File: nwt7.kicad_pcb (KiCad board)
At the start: 2 copper layers, 118.4 x 117.3 mm, 125 parts, among them IC1 PIC16F876A, IC10 AD8307, IC11 MSA0886, IC12 78L10, IC13 AP1117D50, IC15 AP1117D50, IC16 AD8361, IC2 MAX232, IC4 AP1117D50, IC5 AP1117D50, IC6 AD9851, IC7 MSA0886, IC8 7808, IC9 AD8307, Q1 10 MHz, T1 Coupler

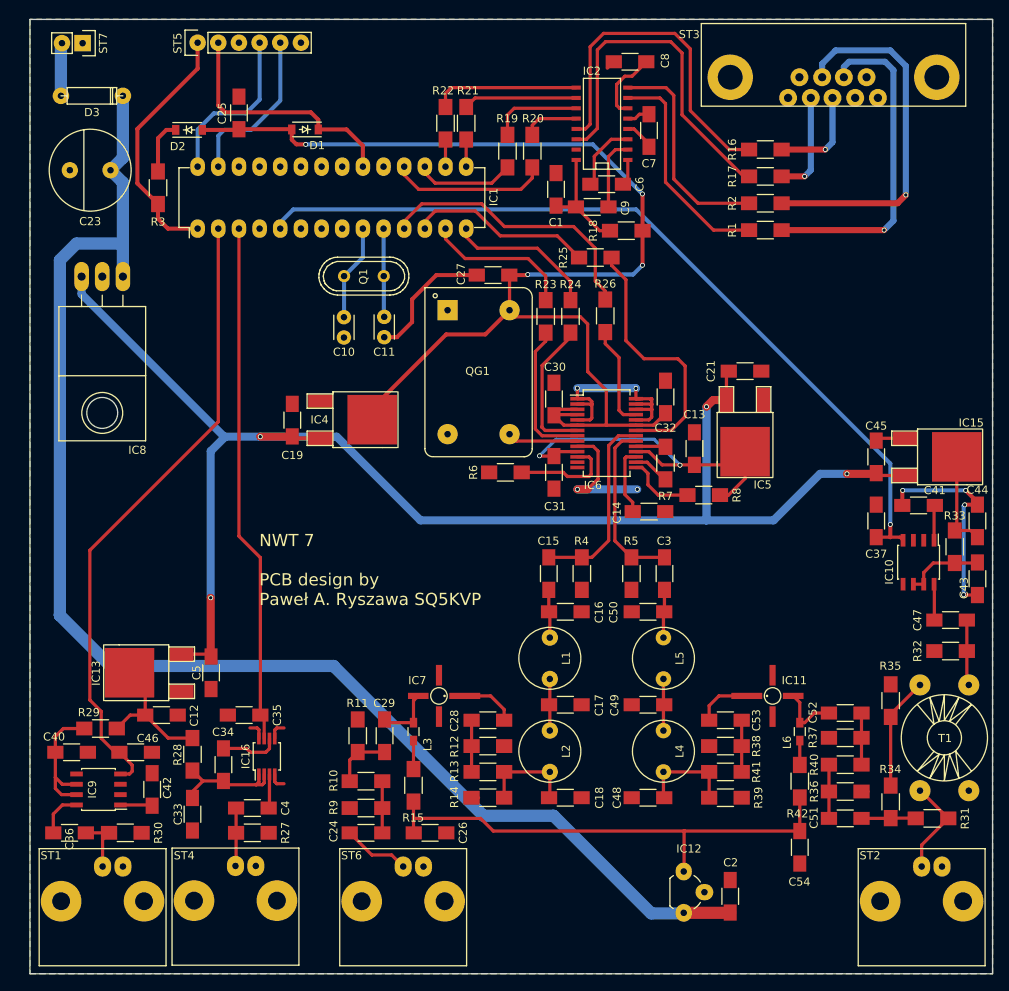
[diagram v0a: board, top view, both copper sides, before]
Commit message: adjusting
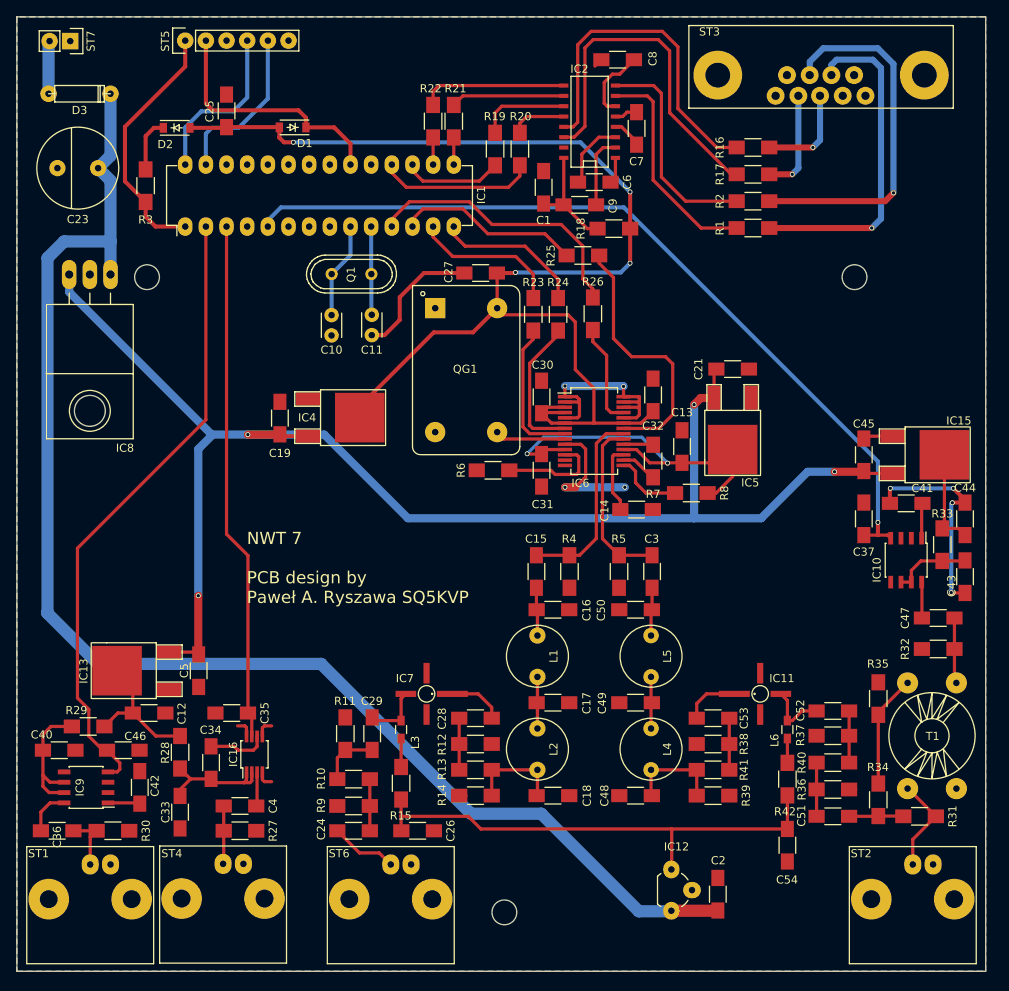
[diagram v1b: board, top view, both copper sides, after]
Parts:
- added REF**: Hole3, DDS:Hole3, F.Cu at (28.1, 44.1)
- added REF**: Hole3, DDS:Hole3, F.Cu at (115.1, 44.1)
- added REF**: Hole3, DDS:Hole3, F.Cu at (72.0, 122.2)
- moved ST3 1.55 mm to (110.8, 20.5)
- moved C15 1.55 mm to (75.9, 80.3)
- moved C16 1.55 mm to (78.0, 85.0)
- moved C17 1.55 mm to (78.0, 96.4)
- moved C18 1.55 mm to (78.0, 107.8)
- moved C19 1.55 mm to (44.4, 61.4)
- moved C28 1.55 mm to (68.5, 98.3)
- moved C3 1.55 mm to (90.2, 80.3)
- moved C31 1.55 mm to (76.6, 67.8)
- moved C32 1.55 mm to (90.3, 58.5)
- moved C34 1.55 mm to (35.9, 103.8)
- moved C35 1.55 mm to (38.5, 97.7)
- moved C40 1.55 mm to (17.3, 102.2)
- moved C42 1.55 mm to (27.2, 106.8)
- moved C43 1.55 mm to (128.7, 80.9)
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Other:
- board size 118.4 x 117.3 mm -> 119.1 x 117.3 mm
